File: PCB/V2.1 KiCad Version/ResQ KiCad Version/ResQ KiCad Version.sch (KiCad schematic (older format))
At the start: 9 parts, among them J1 Spare 1, J2 Spare 2, J3 OLED, J4 SD Card, J5 GPS, J6 Radio, U1 WeMos_D1_mini

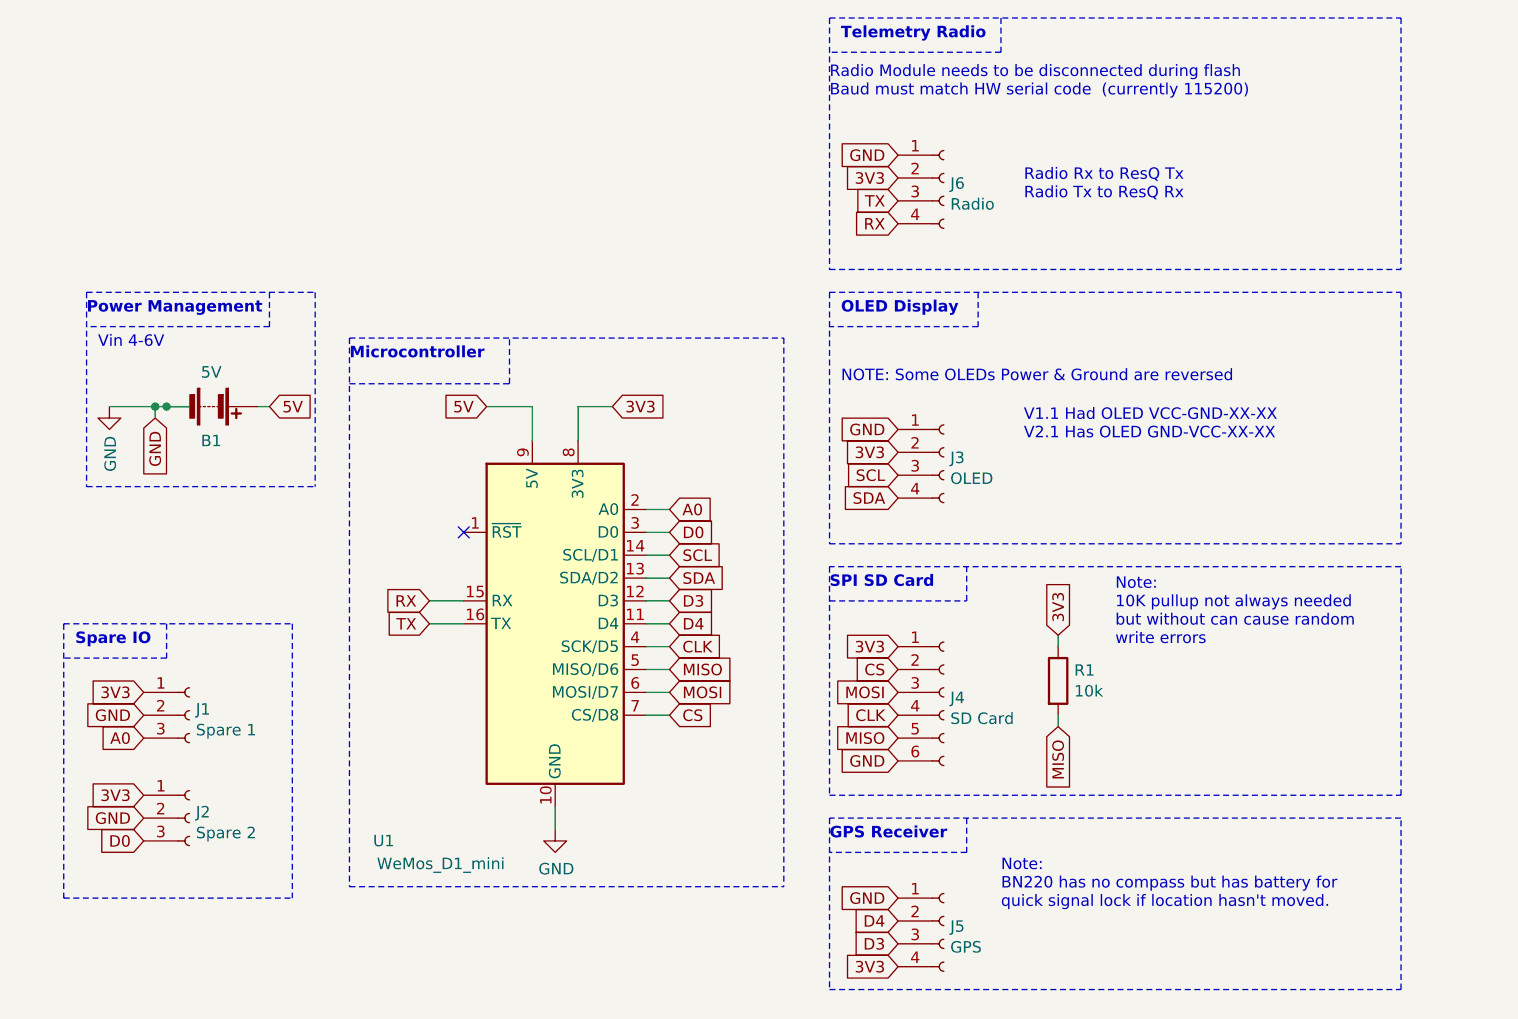
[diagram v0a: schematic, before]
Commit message: Scematic fixes
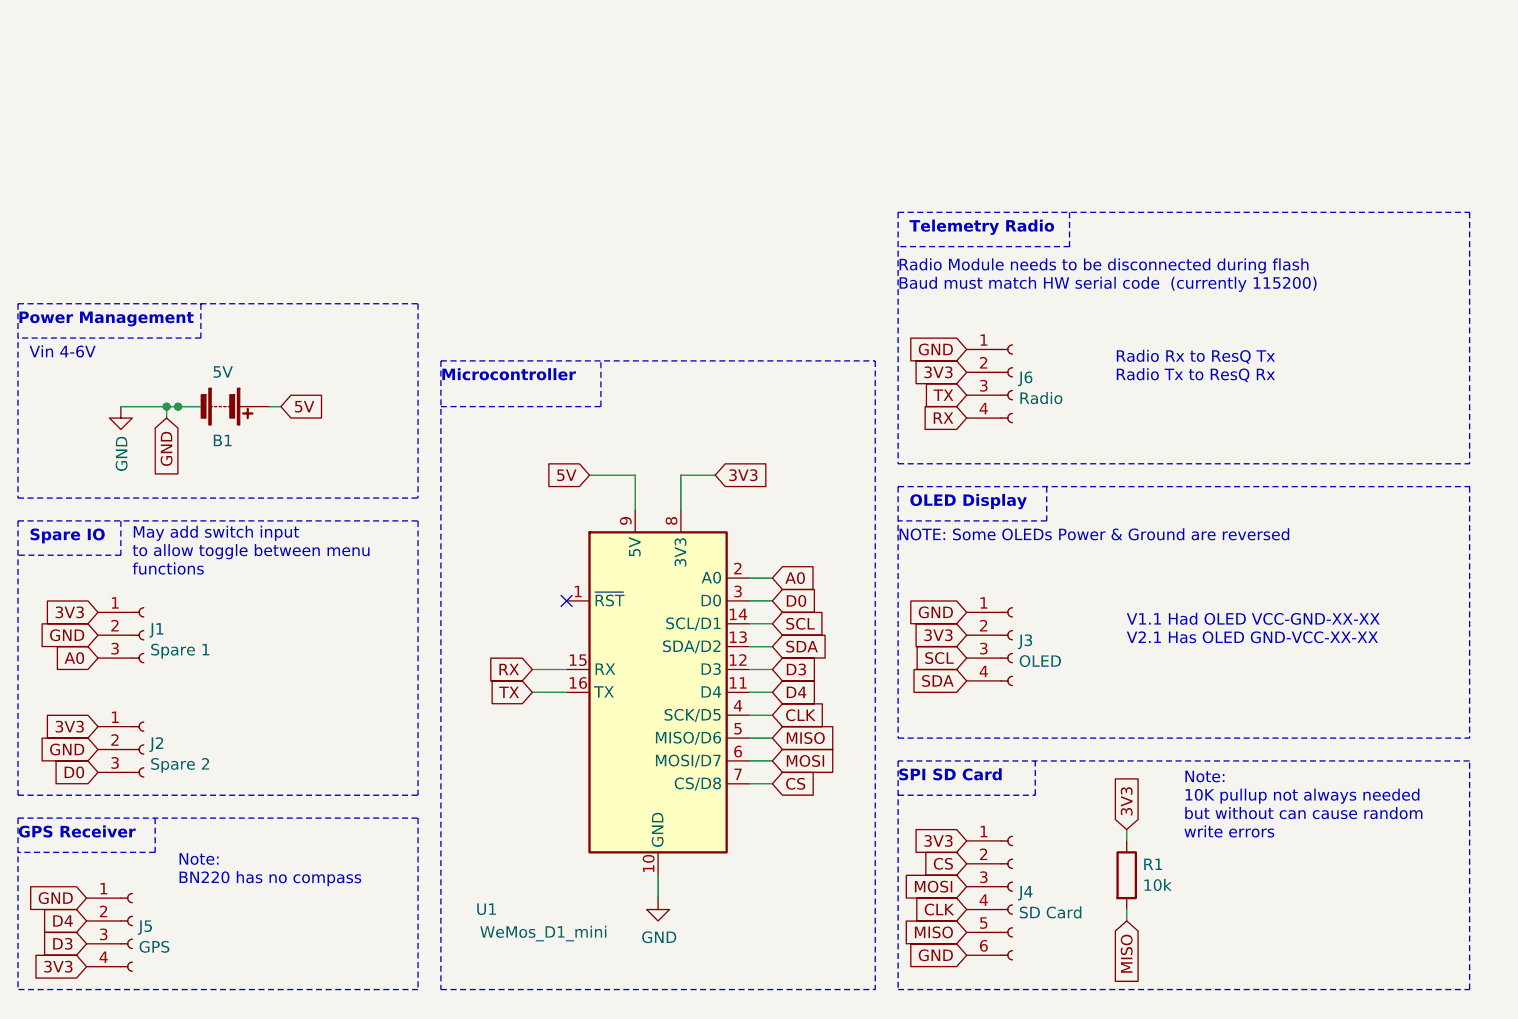
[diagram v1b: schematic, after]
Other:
- note added: "May add switch input\nto allow toggle between menu\nfunctions"
- note added: "Note:\nBN220 has no compass"
- note removed: "Note:\nBN220 has no compass but has battery for \nquick signal lock if location hasn't moved."
- moved on the sheet: B1, J1, J2, J3, J4, J5, J6, R1, U1
